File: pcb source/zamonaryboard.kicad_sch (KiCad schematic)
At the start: 21 parts, among them J1 USB_C_Receptacle_USB2.0_14P, SW1 SW_Push, U1 ESP32-S2, U2 ME6211C33M5, Y1 Crystal_GND24

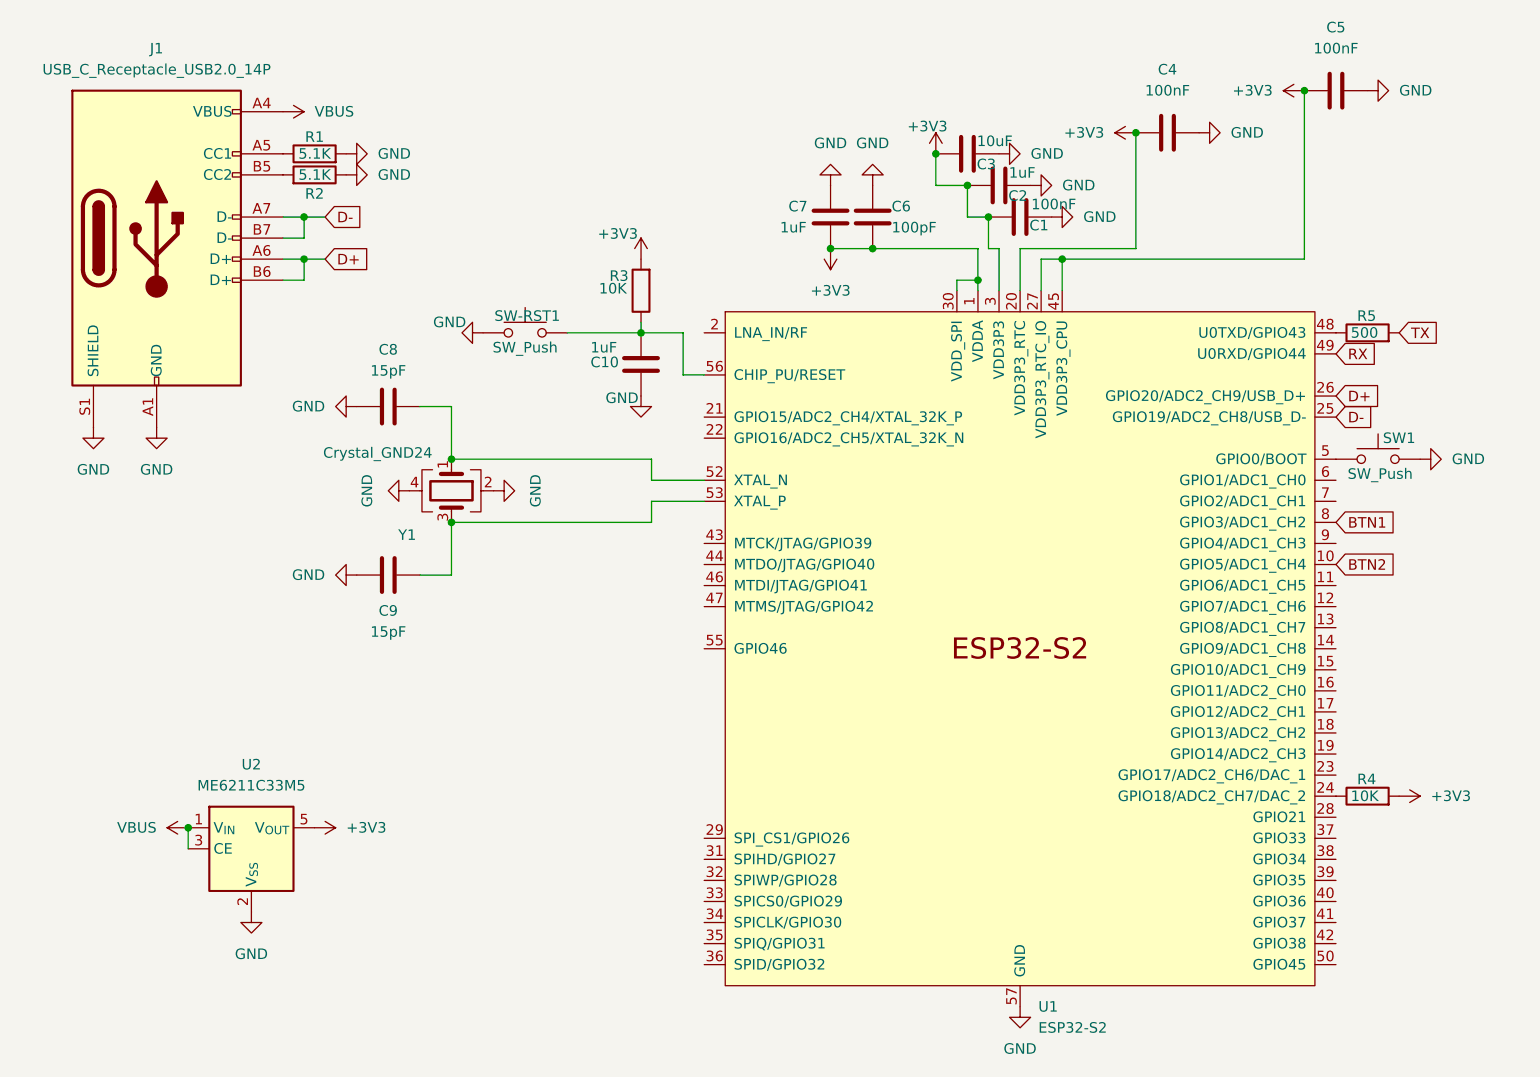
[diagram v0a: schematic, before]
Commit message: v1 commit, desktop app improvements
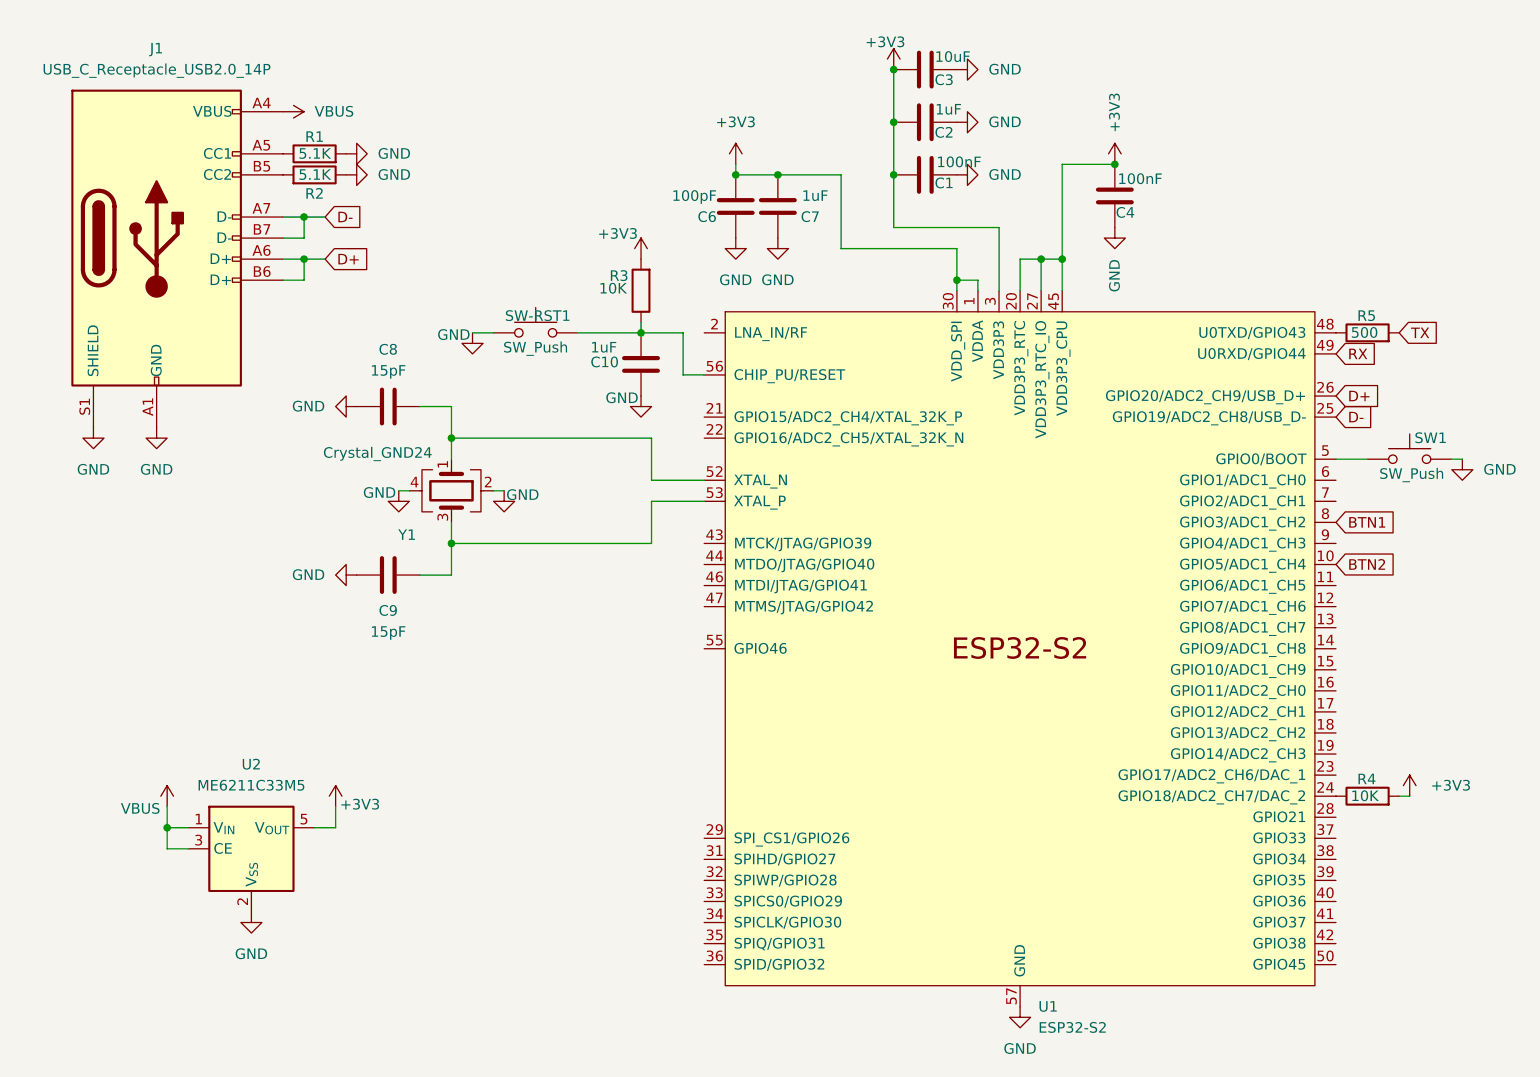
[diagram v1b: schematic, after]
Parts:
- removed C5: 100nF, Capacitor_SMD:C_0603_1608Metric, symbol Device:C
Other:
- moved on the sheet: C1, C2, C3, C4, C6, C7, SW-RST1, SW1
